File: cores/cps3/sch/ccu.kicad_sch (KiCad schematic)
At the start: 1 part, among them J13 DL-2829-CCU

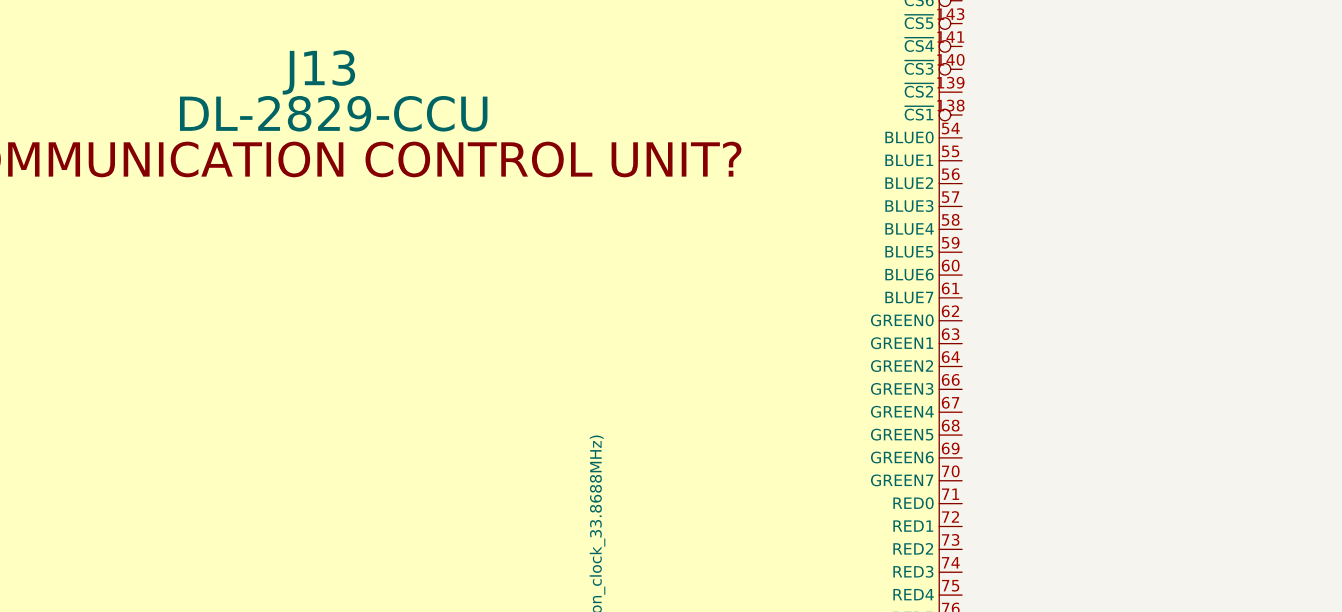
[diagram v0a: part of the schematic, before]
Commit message: update6_cps
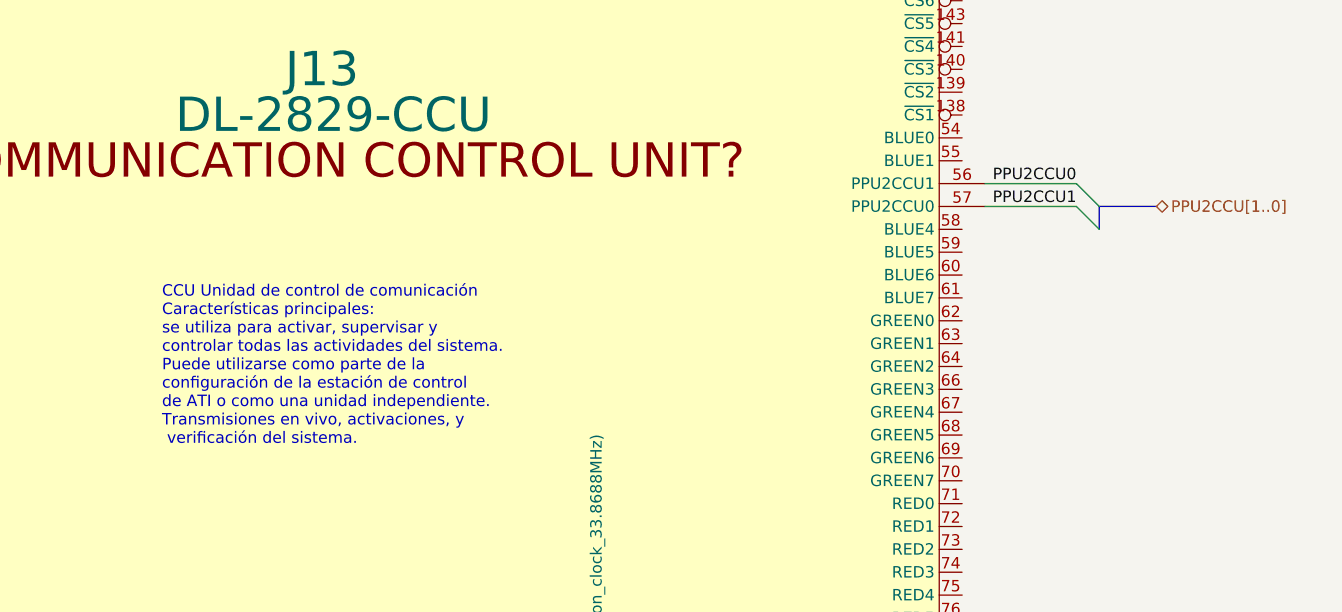
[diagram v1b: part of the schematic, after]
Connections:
- net PPU2CCU0: now reaches J13.56 (PPU2CCU1)
- net PPU2CCU1: now reaches J13.57 (PPU2CCU0)
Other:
- note added: "CCU Unidad de control de comunicación Características principales: se utiliza para activar, supervisar y controlar todas las actividades del sistema. Puede utilizarse como parte de la conﬁguración de la estación de control de ATI o como una unidad independiente. Transmisiones en vivo, activaciones, y veriﬁcación del sistema."
- moved on the sheet: J13
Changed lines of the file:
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@@
     (comment 1 "E.Triana")
+  )
+  (bus_entry (at 284.48 140.97) (size 2.54 2.54)
+    (stroke (width 0) (type default) (color 0 0 0 0))
+  )
+  (bus_entry (at 284.48 138.43) (size 2.54 2.54)
+    (stroke (width 0) (type default) (color 0 0 0 0))
+  )
+  (bus (pts (xy 287.02 140.97) (xy 293.37 140.97))
+    (stroke (width 0) (type default) (color 0 0 0 0))
+  )
+  (wire (pts (xy 274.32 138.43) (xy 284.48 138.43))
+    (stroke (width 0) (type default) (color 0 0 0 0))
+  )
+  (wire (pts (xy 274.32 140.97) (xy 284.48 140.97))
+    (stroke (width 0) (type default) (color 0 0 0 0))
+  )
+  (bus (pts (xy 287.02 143.51) (xy 287.02 140.97))
+    (stroke (width 0) (type default) (color 0 0 0 0))
   )
   (image (at 398.78 261.62) (scale 0.294008)
@@
     )
   )
+  (text "CCU Unidad de control de comunicación \nCaracterísticas principales:\nse utiliza para activar, supervisar y\ncontrolar todas las actividades del sistema.\nPuede utilizarse como parte de la \nconﬁguración de la estación de control \nde ATI o como una unidad independiente. \nTransmisiones en vivo, activaciones, y\n veriﬁcación del sistema.\n"
+    (at 182.88 167.64 0)
+    (effects (font (size 1.27 1.27)) (justify left bottom))
+  )
+  (label "PPU2CCU0" (at 284.48 138.43 180)
+    (effects (font (size 1.27 1.27)) (justify right bottom))
+  )
+  (label "PPU2CCU1" (at 284.48 140.97 180)
+    (effects (font (size 1.27 1.27)) (justify right bottom))
+  )
+  (hierarchical_label "PPU2CCU[1..0]" (shape bidirectional) (at 293.37 140.97 0)
+    (effects (font (size 1.27 1.27)) (justify left))
+  )
   (symbol (lib_id "capcom:DL-2829-CCU") (at 201.93 130.81 0) (unit 1)
